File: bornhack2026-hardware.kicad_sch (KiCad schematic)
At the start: 10 parts, among them J1 USB device

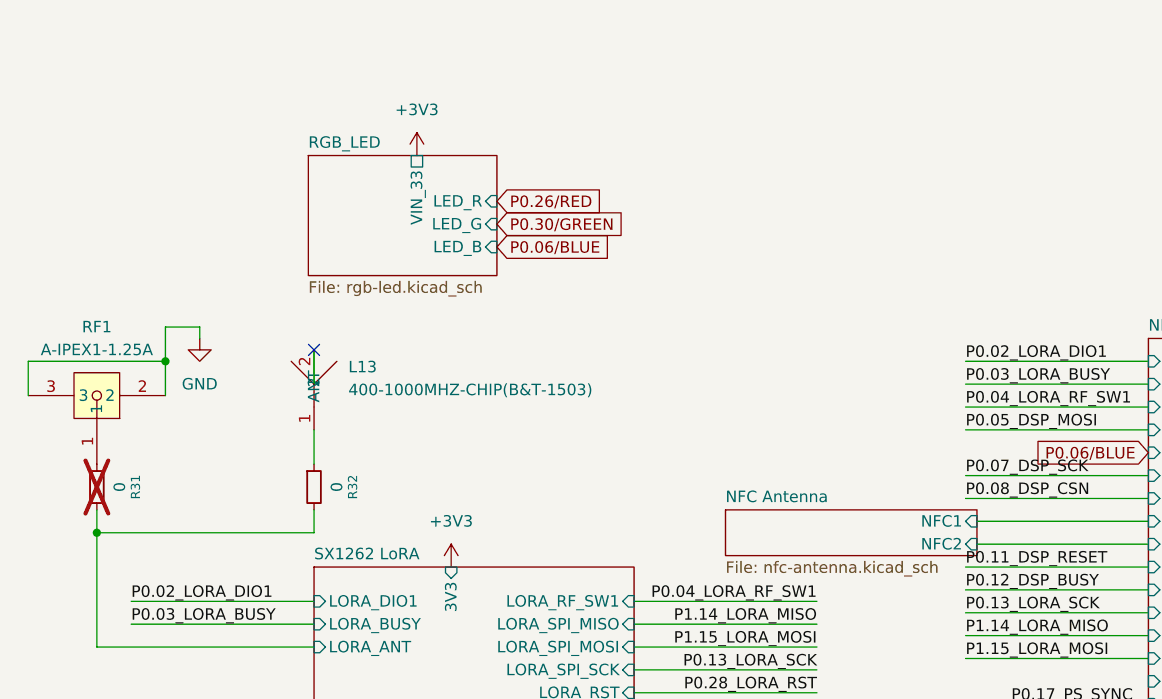
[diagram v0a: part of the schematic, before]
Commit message: Moved SMA-connector Lora for VNA testing.
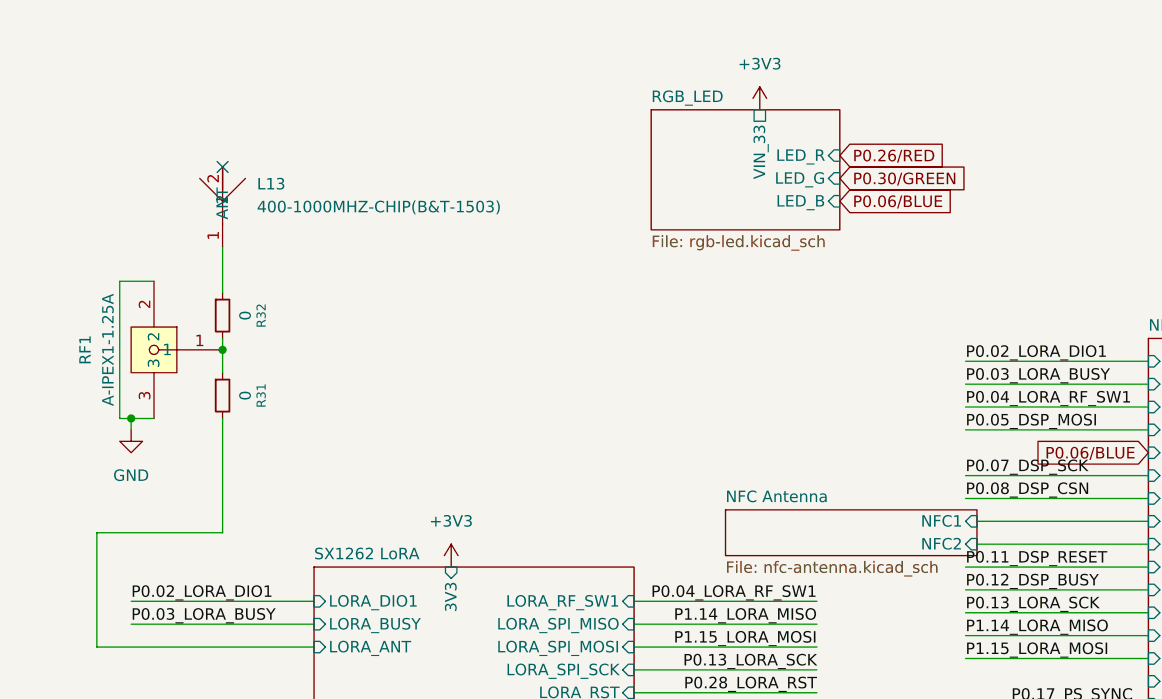
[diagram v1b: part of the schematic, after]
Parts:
- R31: now fitted; now in the parts list
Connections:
- net SX1262 LoRA/LORA_ANT: no longer R32.2
- net at R31.1, RF1.1: now also R32.2
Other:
- moved on the sheet: L13, R32, RF1

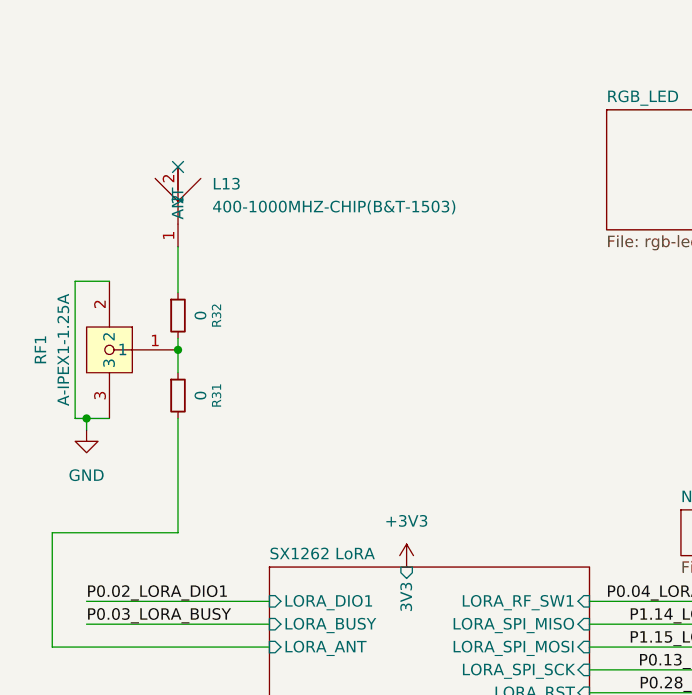
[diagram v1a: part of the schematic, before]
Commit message: WIP: Moved buttons, battery.
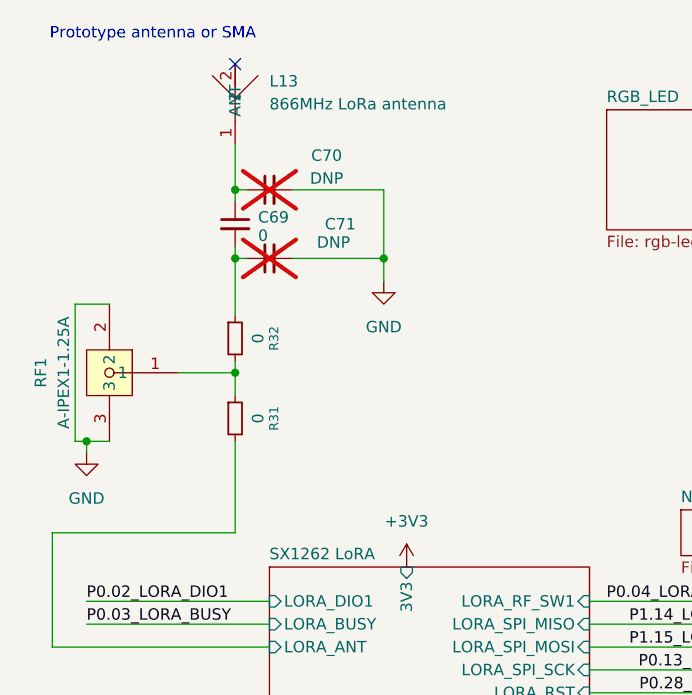
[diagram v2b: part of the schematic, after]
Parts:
- added C69: 0, Capacitor_SMD:C_0402_1005Metric, symbol Device:C_Small
- added C70, C71: DNP, Capacitor_SMD:C_0402_1005Metric, symbol Device:C_Small
- L13: value 400-1000MHZ-CHIP(B&T-1503) -> 866MHz LoRa antenna
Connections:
- net GND: now also C70.2, C71.2
- net at L13.1 (ANT): now also C69.1, C70.1; no longer R32.1
- new net: C69.2, C71.1, R32.1
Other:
- note added: "Prototype antenna or SMA"
- moved on the sheet: L13, R31, R32, RF1
